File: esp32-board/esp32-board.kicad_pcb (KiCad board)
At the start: 2 copper layers, 116.2 x 30 mm, 32 parts, among them J1 remote_header, J3 SOIL_SENSOR, J4 ANT, J5 Conn_01x10_Pin, J6 Conn_01x10_Pin, J7 Battery, SW1 RESET, SW2 ESP Program, SW3 RESET, U1 ESP32-WROOM-32D, U2 XC6220B331MR, U3 XC6220B331MR, U4 TPS3839DBZ, U5 RFM95W-915S2, U6 MAX17048G_T10

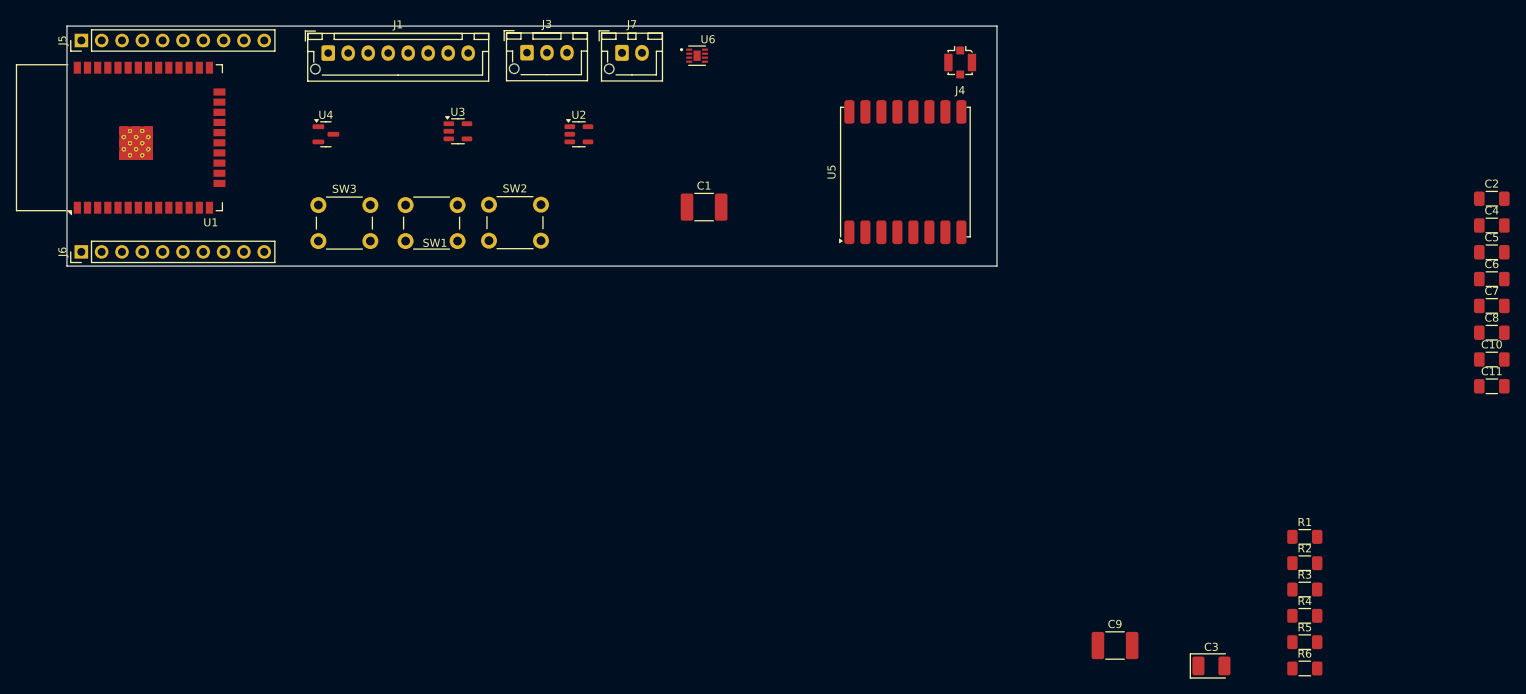
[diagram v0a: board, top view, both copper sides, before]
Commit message: ADD: Final PCB
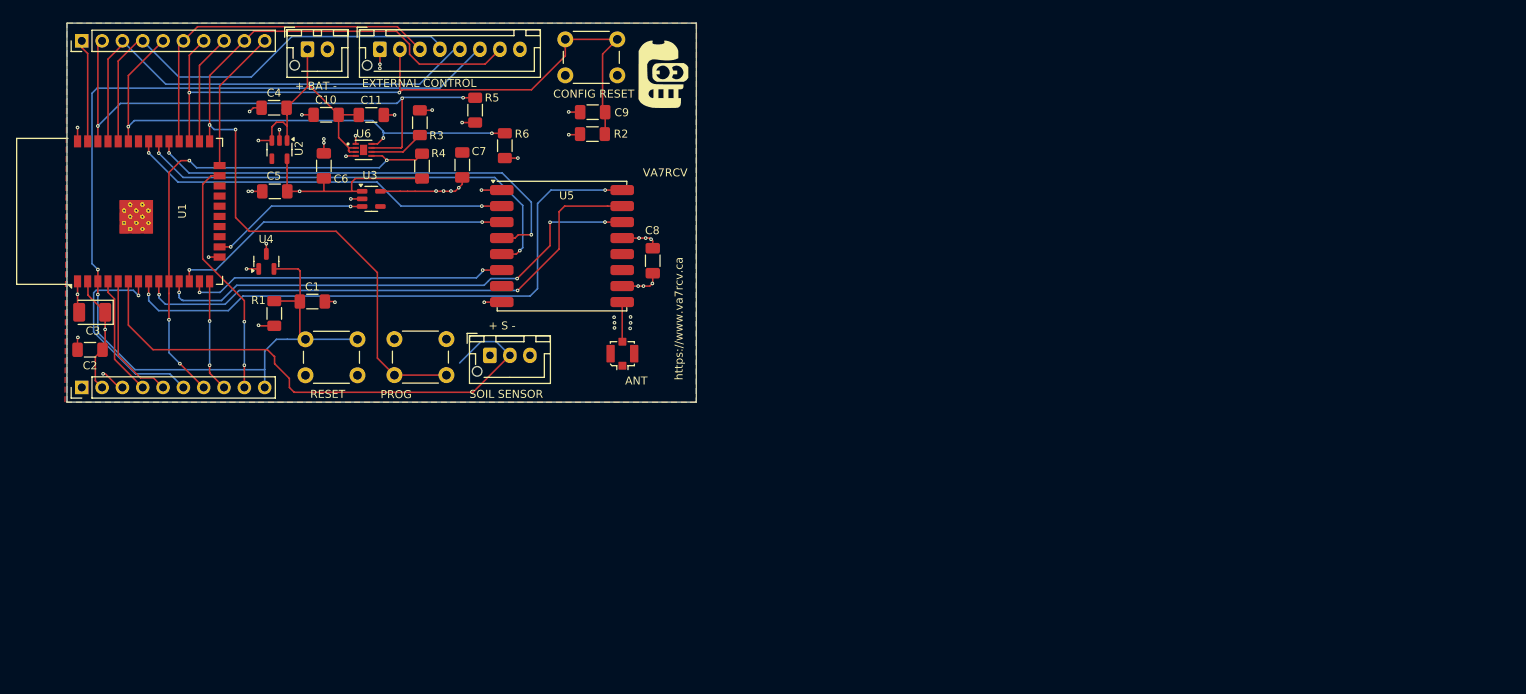
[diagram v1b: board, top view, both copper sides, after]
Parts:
- added G***: LOGO, LOGO:logo, F.Cu at (152.2, 63.9)
- added G***: LOGO, LOGO:logo, B.Cu at (152.6, 64.1)
- + BAT -: renamed from J7
- C1, C9: footprint Capacitor_SMD:C_1812_4532Metric_Pad1.57x3.40mm_HandSolder -> Capacitor_SMD:C_1206_3216Metric_Pad1.33x1.80mm_HandSolder
- CONFIG RESET: renamed from SW3; value RESET -> WEB_CONF
- EXTERNAL CONTROL: renamed from J1
- SOIL SENSOR: renamed from J3
- moved C2 176.2 mm to (80.9, 98.5), turned to 180 degrees
- moved C4 152.9 mm to (103.9, 68.2), turned to 180 degrees
- moved C5 152.3 mm to (104.0, 78.7), turned to 180 degrees
- moved C10 148.9 mm to (110.4, 69.1)
- moved C3 146.7 mm to (81.1, 93.8), turned to 180 degrees
- moved C6 146.7 mm to (110.1, 75.5), turned to -90 degrees
- moved C11 144.1 mm to (116.0, 69.1)
- moved R1 131.8 mm to (103.9, 93.9), turned to 90 degrees
- moved C7 129.9 mm to (127.4, 75.4), turned to 90 degrees
- moved R3 125.1 mm to (122.1, 70.1), turned to -90 degrees
- moved R4 123.8 mm to (122.4, 75.5), turned to 90 degrees
- moved R5 123.2 mm to (129.0, 68.5), turned to 90 degrees
- moved R6 119.5 mm to (132.7, 73.0), turned to 90 degrees
- moved C8 105.3 mm to (151.2, 87.3), turned to 90 degrees
- moved R2 104.0 mm to (143.7, 71.5)
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- renumbered J4 to ANT, SW2 to PROG, SW1 to RESET
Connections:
- EXTERNAL CONTROL pad 4: ESP_TX -> ESP_RX
- EXTERNAL CONTROL pad 5: ESP_RX -> ESP_TX
- J5 pad 1: ESP_PROG -> GPIO23
- J5 pad 10: GPIO_15 -> GPIO02
- J5 pad 2: ESP_ENA -> I2C_SCL
- J5 pad 3: GND -> ESP_TX
- J5 pad 4: VCC -> ESP_RX
- J5 pad 5: VCC_AUX -> I2C_SDA
- J5 pad 6: START_WEB_CONFIG -> LED_DATA_PIN
- J5 pad 7: GPIO02 -> START_WEB_CONFIG
- J5 pad 9: GPIO_12 -> ESP_PROG
- J6 pad 1: GPIO_17 -> GND
- J6 pad 10: ESP_RX -> ESP_ENA
- J6 pad 2: I2C_SDA -> VCC
- J6 pad 3: I2C_SCL -> VCC_AUX
- J6 pad 4: GPIO23 -> SENSOR_VP
- J6 pad 5: BAT_ALERT -> SENSOR_VN
- J6 pad 7: SENSOR_VN -> BAT_ALERT
- J6 pad 8: SENSOR_VP -> GPIO_12
- J6 pad 9: ESP_TX -> GPIO_15
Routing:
- net ESP_ENA: track 0.00 -> 136.0 mm, vias 0 -> 2
- net ESP_PROG: track 0.00 -> 105.6 mm, vias 0 -> 2
- net START_WEB_CONFIG: track 0.00 -> 88.6 mm, vias 0 -> 2
- net VCC: track 0.00 -> 86.1 mm, vias 0 -> 3
- net LORA_DIO2: track 0.00 -> 74.6 mm, vias 0 -> 2
- net I2C_SCL: track 0.00 -> 71.8 mm, vias 0 -> 3
- net LORA_DIO1: track 0.00 -> 68.1 mm, vias 0 -> 2
- net SOIL_SENSOR: track 0.00 -> 67.8 mm
- net I2C_SDA: track 0.00 -> 65.2 mm, vias 0 -> 3
- net BAT_ALERT: track 0.00 -> 64.2 mm, vias 0 -> 4
- net LORA_DIO0: track 0.00 -> 63.3 mm, vias 0 -> 4
- net ESP_TX: track 0.00 -> 59.4 mm
- net LORA_NSS: track 0.00 -> 57.9 mm, vias 0 -> 2
- net LORA_SCK: track 0.00 -> 57.2 mm, vias 0 -> 2
- net ESP_RX: track 0.00 -> 56.5 mm
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- added copper zone on B.Cu, net GND
- added copper zone on F.Cu, net GND
- added copper zone on In1.Cu, net GND
- added copper zone on In2.Cu, net VCC_AUX
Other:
- board size 116.2 x 30 mm -> 78.7 x 47.4 mm
- copper layers 2 -> 4
- board text added: "+ BAT -"
- board text added: "+ S -"
- board text added: "BAT_ALERT"
- board text added: "GND"
- board text added: "GPIO02"
- board text added: "GPIO04"
- board text added: "GPIO15"
- board text added: "GPIO22"
- board text added: "GPIO23"
- board text added: "GPIO35"
- board text added: "LED_DATA"
- board text added: "PROG"
- board text added: "RESET"
- board text added: "RX"
- board text added: "SCL"
- board text added: "SDA"
- board text added: "SENSOR_VN"
- board text added: "SENSOR_VP"
- board text added: "TX"
- board text added: "VA7RCV"
- board text added: "VCC"
- board text added: "VCC_AUX"
- board text added: "WEB_CONFIG"
- board text added: "https://www.va7rcv.ca"
